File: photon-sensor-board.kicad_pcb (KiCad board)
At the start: 2 copper layers, 35 x 50 mm, 6 parts, among them M1 MountingHole_2-5mm, M2 MountingHole_2-5mm, U1 PHOTON, U2 DS18B20

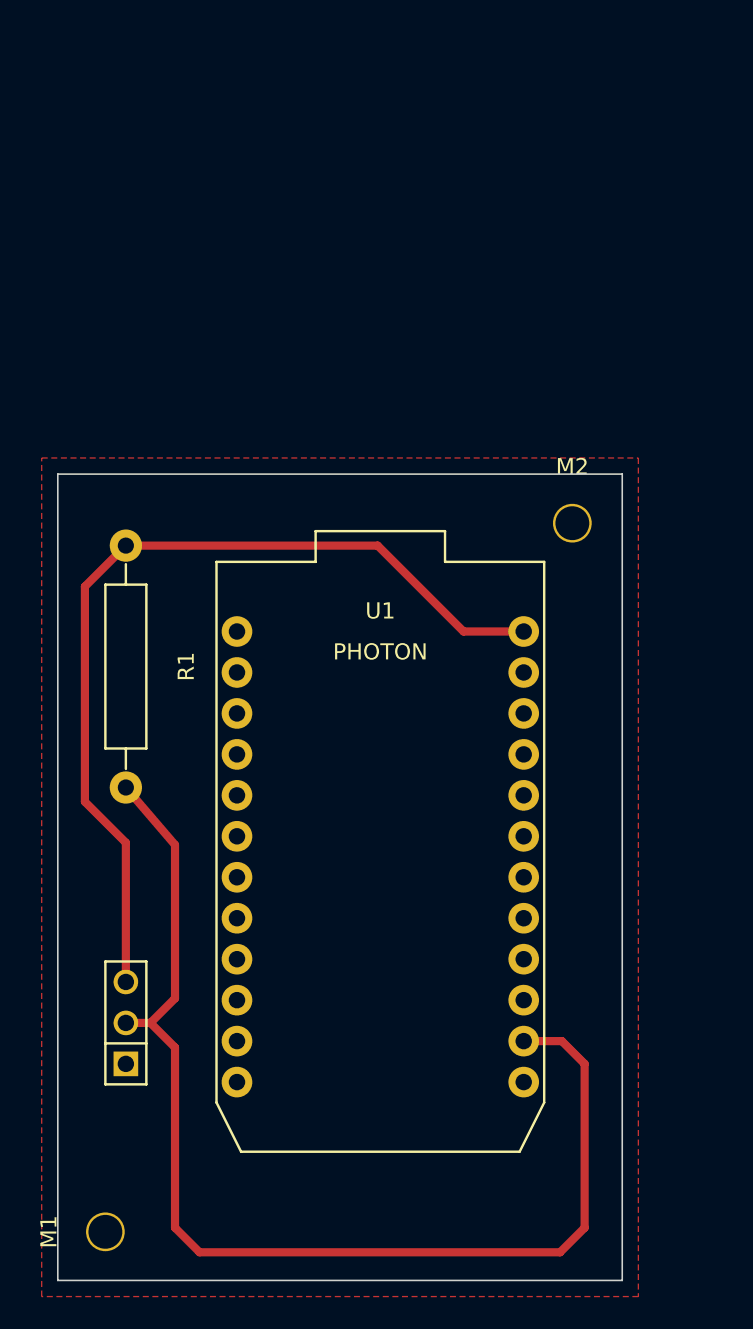
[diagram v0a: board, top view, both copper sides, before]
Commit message: Some adjustments
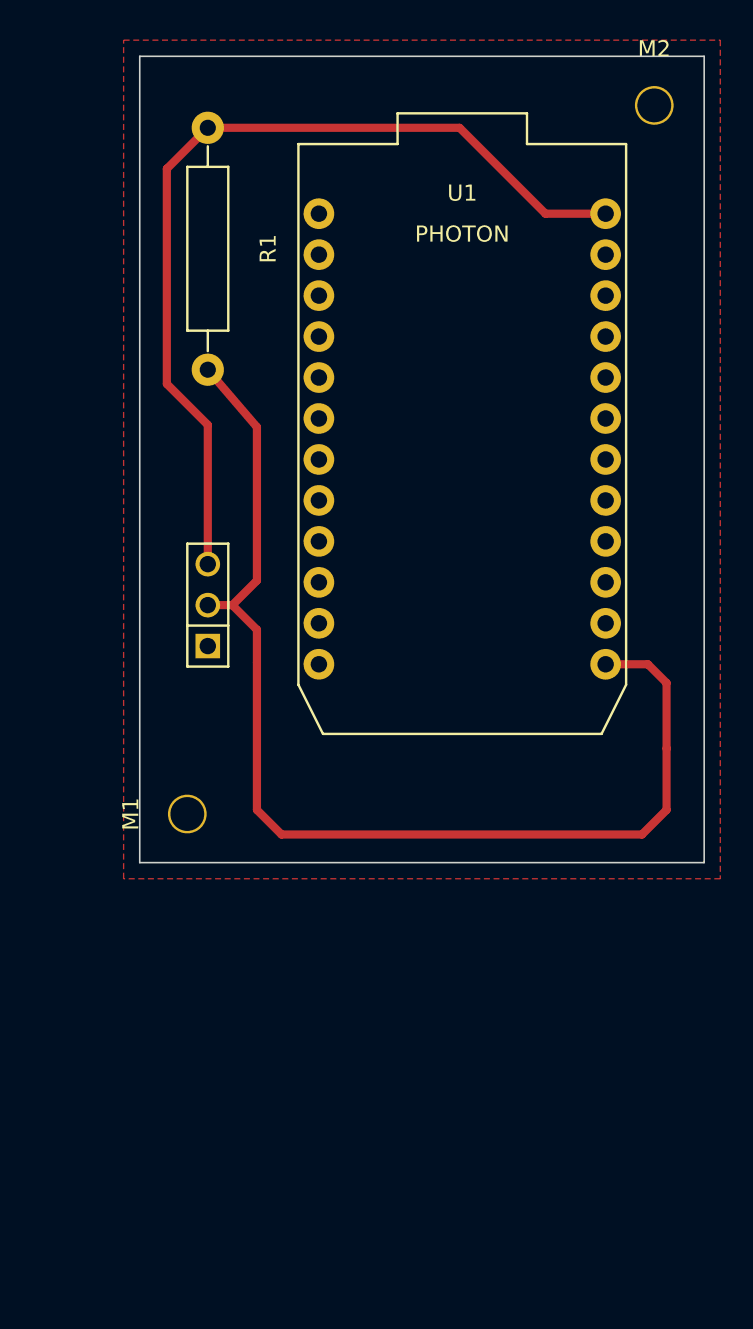
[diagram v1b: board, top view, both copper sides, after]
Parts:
- moved U2 26.4 mm to (114.3, 103.1)
- moved G*** 26.4 mm to (130.1, 88.1)
- moved R1 26.4 mm to (114.3, 81.0)
- moved U1 26.4 mm to (130.1, 94.1)
- moved M2 26.4 mm to (142.0, 72.1)
- moved M1 26.4 mm to (113.0, 116.1)
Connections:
- U1 pad 13: Net-(U1-Pad13) -> Net-(R1-Pad2)
- U1 pad 14: Net-(R1-Pad2) -> Net-(U1-Pad14)
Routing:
- net Net-(R1-Pad2): track 72.6 -> 70.0 mm
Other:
- board text added: "Photon Sensor Board v1.1 2015"
